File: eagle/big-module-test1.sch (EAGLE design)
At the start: 4 parts

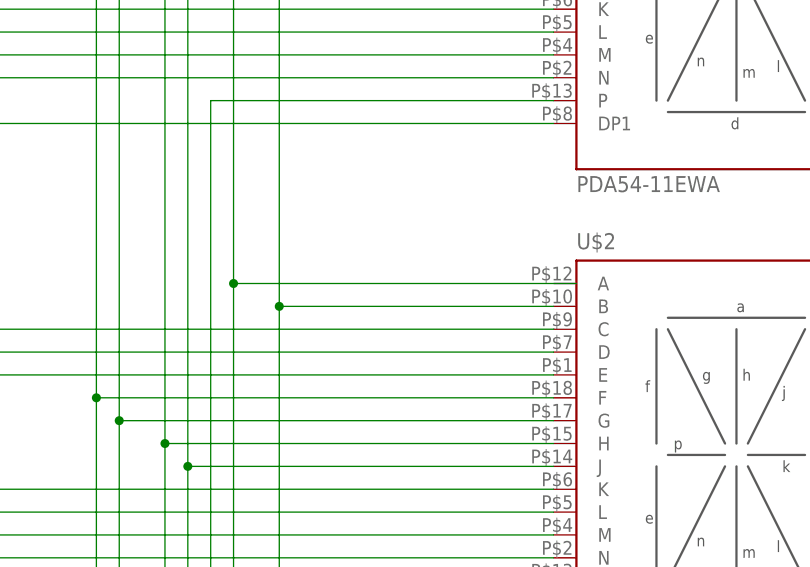
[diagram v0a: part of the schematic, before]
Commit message: new boards and source code
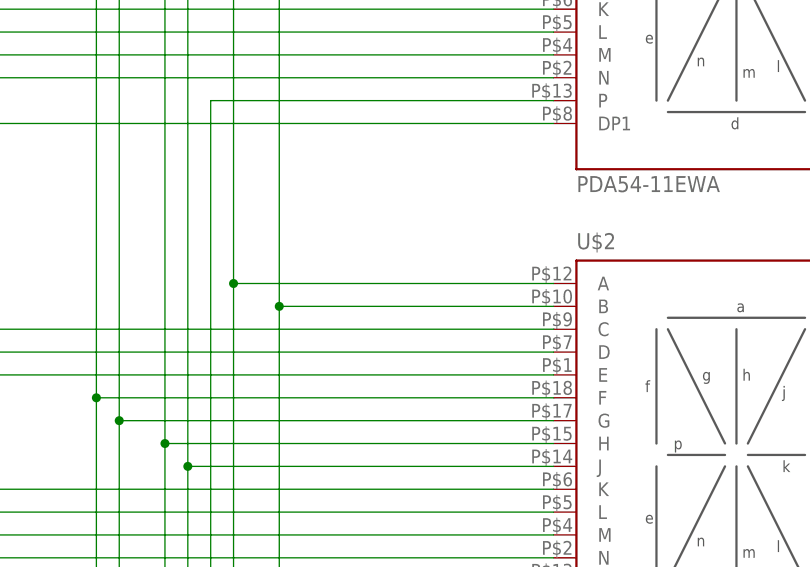
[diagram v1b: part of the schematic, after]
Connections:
- net N$15: now also U$2.A
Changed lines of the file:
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@@
 <wire x1="86.36" y1="134.62" x2="86.36" y2="81.28" width="0.1524" layer="91"/>
 <wire x1="86.36" y1="81.28" x2="86.36" y2="7.62" width="0.1524" layer="91"/>
-<wire x1="124.46" y1="81.28" x2="86.36" y2="81.28" width="0.1524" layer="91"/>
+<wire x1="121.92" y1="81.28" x2="86.36" y2="81.28" width="0.1524" layer="91"/>
 <junction x="86.36" y="81.28"/>
 <pinref part="SV2" gate="1" pin="4"/>
+<pinref part="U$2" gate="G$1" pin="A"/>
 </segment>
 </net>
